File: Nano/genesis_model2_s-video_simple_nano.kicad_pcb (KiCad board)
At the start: 2 copper layers, 16 x 8.2 mm, 10 parts, among them J1 Y In, J2 C In, J3 Y Out, J4 C Out, J5 GND, J6 GND

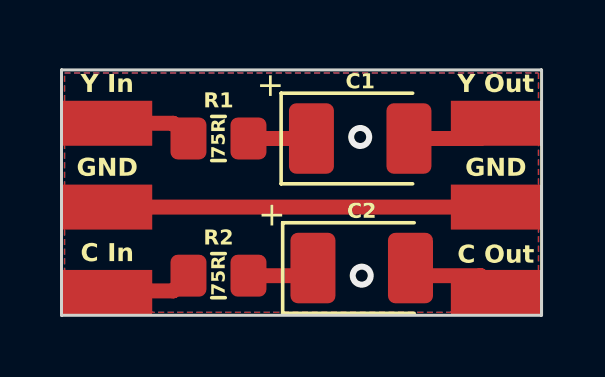
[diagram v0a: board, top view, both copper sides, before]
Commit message: nano - minor update
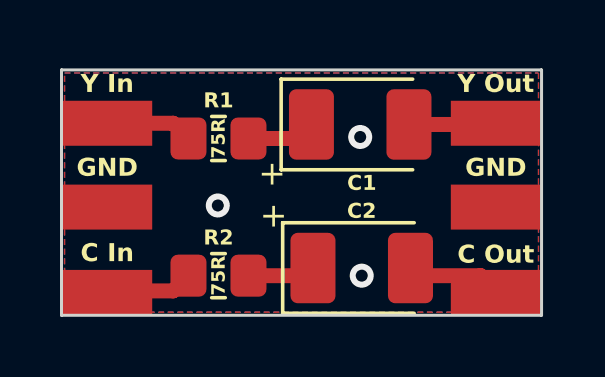
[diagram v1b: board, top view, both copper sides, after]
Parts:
- moved C1 0.47 mm to (114.1, 73.7)
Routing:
- net GND: track 13.0 -> 0.00 mm, vias 2 -> 3
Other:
- board text removed: "Y = Luma C = Chroma"
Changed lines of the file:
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@@
   )
   (footprint "Capacitor_Tantalum_SMD:CP_EIA-3528-15_AVX-H_Pad1.50x2.35mm_HandSolder" (layer "F.Cu")
-    (at 114.0968 74.168)
+    (at 114.0968 73.7)
     (descr "Tantalum Capacitor SMD AVX-H (3528-15 Metric), IPC_7351 nominal, (Body size from: http://www.kemet.com/Lists/ProductCatalog/Attachments/253/KEM_TC101_STD.pdf), generated with kicad-footprint-generator")
     (tags "capacitor tantalum")
@@
     (property "ki_keywords" "cap capacitor")
     (attr smd)
-    (fp_text reference "C1" (at 0 -1.905) (layer "F.SilkS")
+    (fp_text reference "C1" (at 0.0532 1.95) (layer "F.SilkS")
         (effects (font (size 0.5 0.5) (thickness 0.1) bold))
     )
@@
   (gr_rect (start 104.14 71.882) (end 120.142 80.0608)
     (stroke (width 0.1) (type default)) (fill none) (layer "Edge.Cuts"))
-  (gr_text "Y = Luma\nC = Chroma" (at 109.5248 79.883) (layer "B.SilkS")
-    (effects (font (size 0.55 0.55) (thickness 0.1) bold) (justify left bottom mirror))
-  )
   (gr_text "Model 2&3 MD/SG S-Video\nBy joshman196" (at 120.015 73.787) (layer "B.SilkS")
     (effects (font (size 0.6 0.6) (thickness 0.1) bold) (justify left bottom mirror))
   )
-  (gr_text "JLCJLCJLCJLC" (at 116.332 76.8096) (layer "B.SilkS")
-    (effects (font (size 0.8 0.8) (thickness 0.15)) (justify left bottom mirror))
-  )
-  (gr_text "+" (at 110.6932 77.1652) (layer "F.SilkS")
+  (gr_text "JLCJLCJLCJLC" (at 120.05 80) (layer "B.SilkS")
+    (effects (font (size 0.7 0.7) (thickness 0.1)) (justify left bottom mirror))
+  )
+  (gr_text "+" (at 110.75 77.2) (layer "F.SilkS")
     (effects (font (size 0.8 0.8) (thickness 0.15)) (justify left bottom))
   )
-  (gr_text "+" (at 110.6424 72.8472) (layer "F.SilkS")
+  (gr_text "+" (at 110.7 75.8) (layer "F.SilkS")
     (effects (font (size 0.8 0.8) (thickness 0.15)) (justify left bottom))
   )
-  (segment (start 110.3724 74.168) (end 112.4718 74.168) (width 0.5) (layer "F.Cu") (net 1))
-  (segment (start 115.7218 74.168) (end 118.11 74.168) (width 0.5) (layer "F.Cu") (net 2))
-  (segment (start 118.11 74.168) (end 118.618 73.66) (width 0.5) (layer "F.Cu") (net 2))
+  (segment (start 112.0038 74.168) (end 112.4718 73.7) (width 0.5) (layer "F.Cu") (net 1))
+  (segment (start 110.3724 74.168) (end 112.0038 74.168) (width 0.5) (layer "F.Cu") (net 1))
+  (segment (start 118.578 73.7) (end 118.618 73.66) (width 0.5) (layer "F.Cu") (net 2))
+  (segment (start 115.7218 73.7) (end 118.578 73.7) (width 0.5) (layer "F.Cu") (net 2))
   (segment (start 110.3724 78.74) (end 112.522 78.74) (width 0.5) (layer "F.Cu") (net 3))
   (segment (start 118.11 78.74) (end 118.618 79.248) (width 0.5) (layer "F.Cu") (net 4))
@@
   (segment (start 107.8644 79.248) (end 108.3724 78.74) (width 0.5) (layer "F.Cu") (net 6))
   (segment (start 105.664 79.248) (end 107.8644 79.248) (width 0.5) (layer "F.Cu") (net 6))
-  (segment (start 105.664 76.454) (end 118.618 76.454) (width 0.5) (layer "F.Cu") (net 7))
   (via (at 114.0968 74.1172) (size 0.8) (drill 0.4) (layers "F.Cu" "B.Cu") (free) (net 7))
   (via (at 114.1476 78.74) (size 0.8) (drill 0.4) (layers "F.Cu" "B.Cu") (free) (net 7))
+  (via (at 109.35 76.4) (size 0.8) (drill 0.4) (layers "F.Cu" "B.Cu") (free) (net 7))
   (zone (net 7) (net_name "GND") (layers "F&B.Cu") (hatch edge 0.5)
-    (connect_pads (clearance 0.5))
+    (connect_pads (clearance 0.25))
     (min_thickness 0.25) (filled_areas_thickness no)
     (fill yes (thermal_gap 0.5) (thermal_bridge_width 0.5))
